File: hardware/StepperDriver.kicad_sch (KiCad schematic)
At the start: 17 parts, among them J201 Conn_01x01, J202 Conn_01x01, J203 Conn_01x01, J204 Conn_01x01, U201 TMC2130-LA

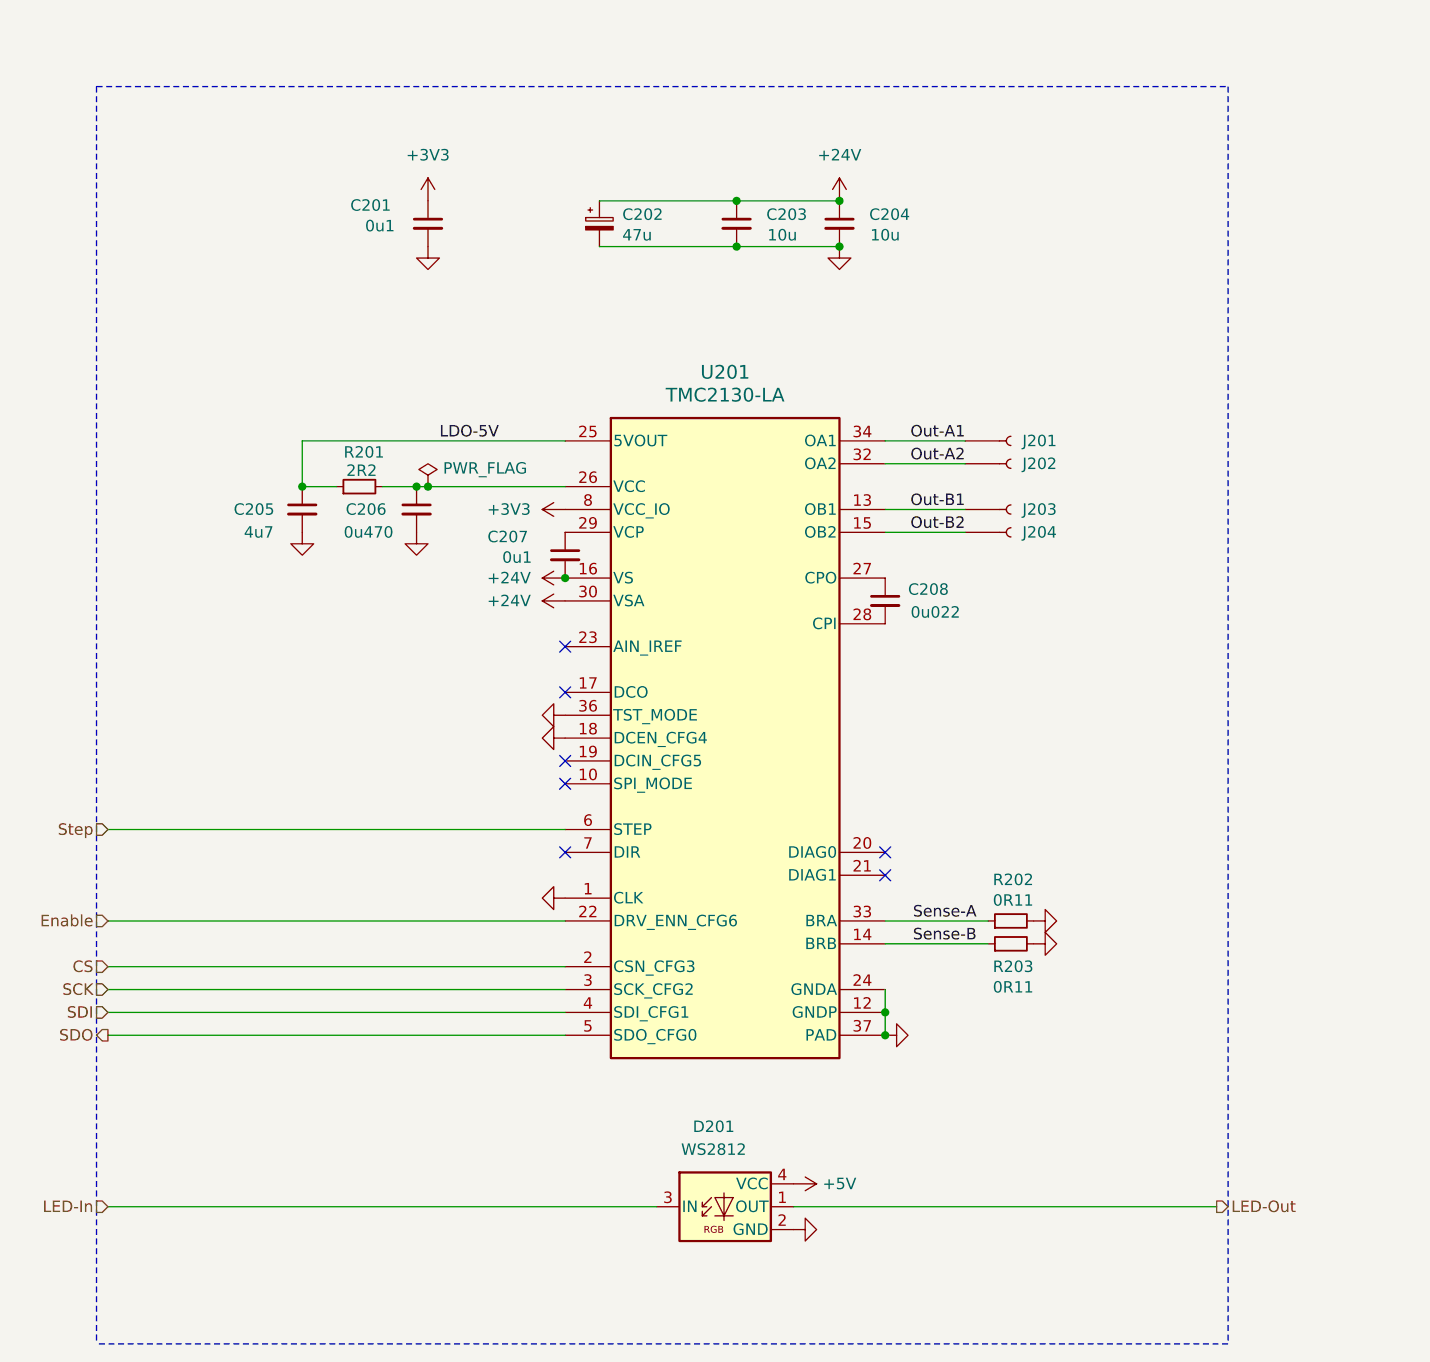
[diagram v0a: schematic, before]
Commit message: Update parts library
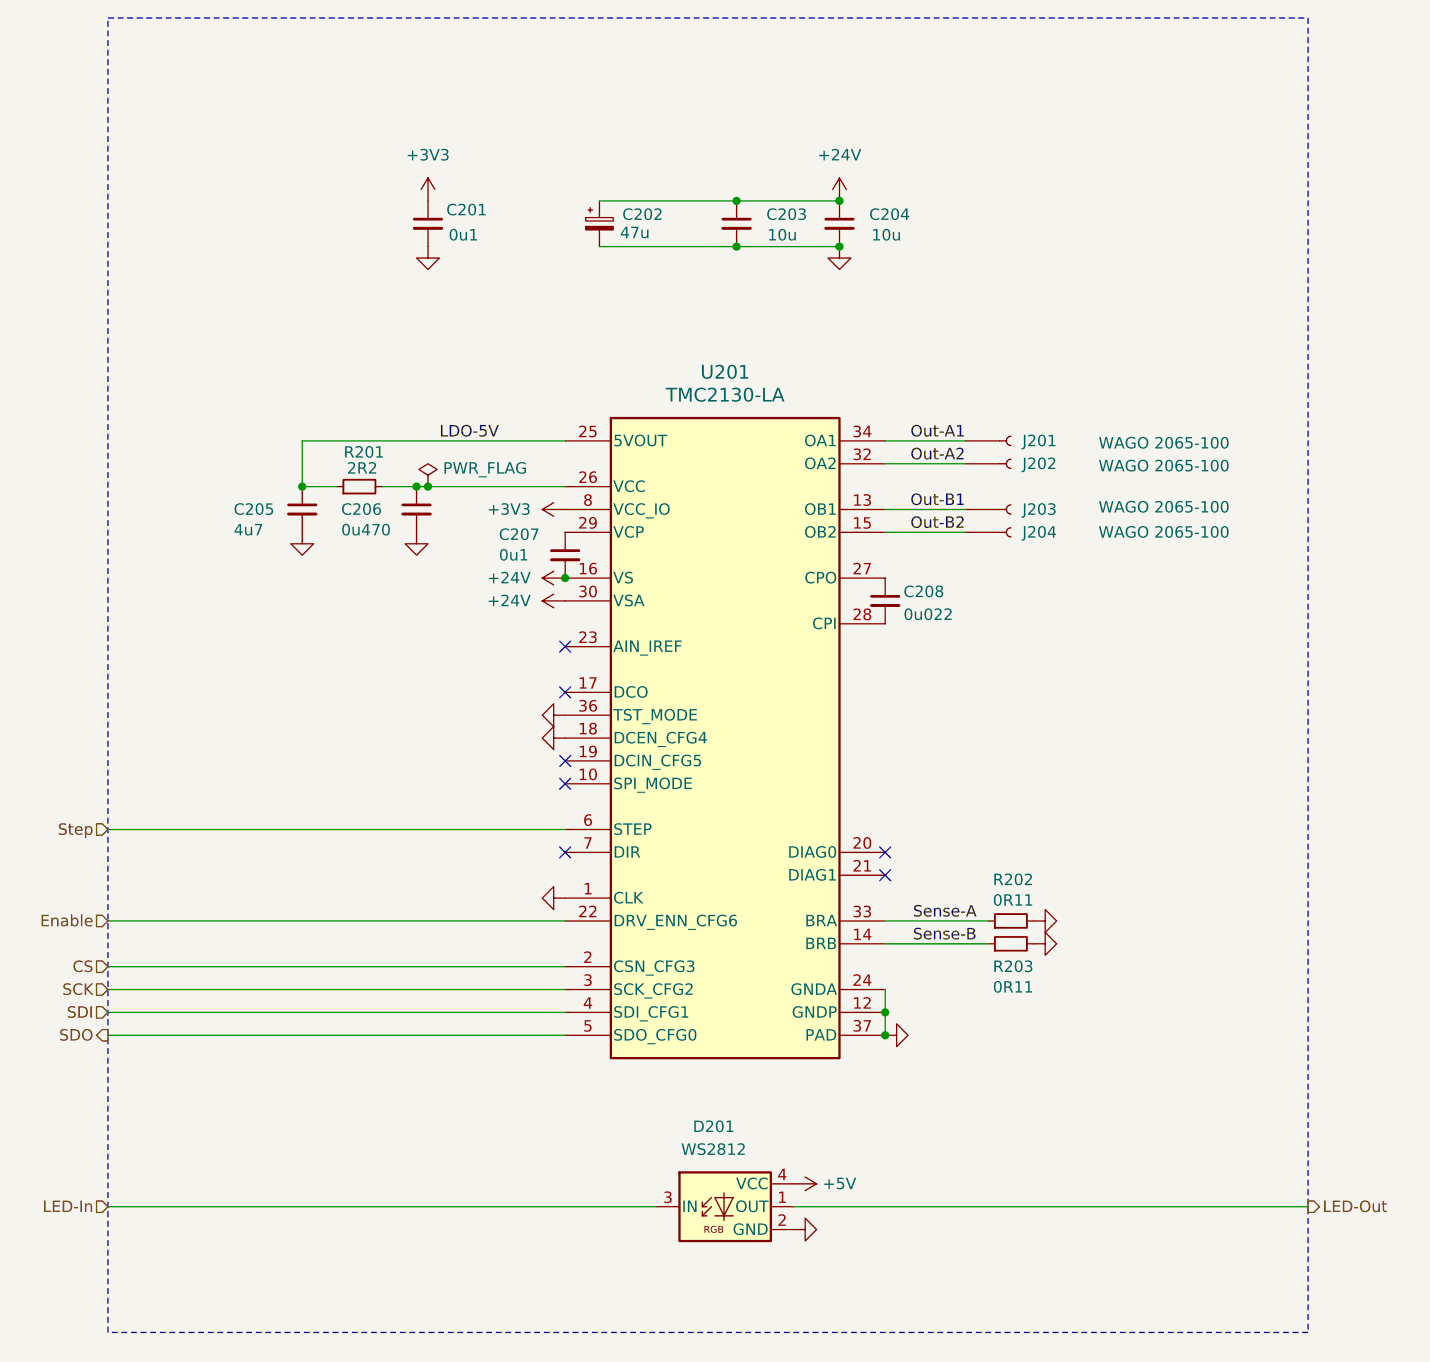
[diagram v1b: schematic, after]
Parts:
- C201, C207: footprint Capacitor_SMD:C_0603_1608Metric -> V2_Capacitor_SMD:C_0603; symbol Device:C_Small -> V2_Device:C_0603_0u1; Mouser (none) -> 810-CGA3E2X7R1H104MA
- C202: footprint Capacitor_SMD:CP_Elec_6.3x5.8 -> V2_Capacitor_SMD:CP_Elec_6.3x5.8; symbol Device:C_Polarized_Small -> V2_Device:C_Polarized_6.3x5.8_1_47u; Mouser (none) -> 667-EEE-FK1V470P
- C203, C204: footprint Capacitor_SMD:C_1210_3225Metric -> V2_Capacitor_SMD:C_1210; symbol Device:C_Small -> V2_Device:C_1210_10u; Mouser (none) -> 810-CNA6P1X7R1H106K2; Rating (none) -> 50V
- C205: footprint Capacitor_SMD:C_0603_1608Metric -> V2_Capacitor_SMD:C_0603; symbol Device:C_Small -> V2_Device:C_0603_4u7; Mouser (none) -> 603-CC603KRX5R6BB475
- C206: footprint Capacitor_SMD:C_0603_1608Metric -> V2_Capacitor_SMD:C_0603; symbol Device:C_Small -> V2_Device:C_0603_0u470; Mouser (none) -> 603-CC0603JR6BB474
- C208: footprint Capacitor_SMD:C_0603_1608Metric -> V2_Capacitor_SMD:C_0603; symbol Device:C_Small -> V2_Device:C_0603_0u022; Mouser (none) -> 603-CC603KPX7R9BB223
- J201, J202, J203, J204: value Conn_01x01 -> WAGO 2065-100
- R201: footprint Resistor_SMD:R_0603_1608Metric -> V2_Resistor_SMD:R_0603; symbol Device:R_Small -> V2_Device:R_0603_2R2; Mouser (none) -> 71-RCS06032R20JNEA
- R202, R203: footprint Resistor_SMD:R_0805_2012Metric -> V2_Resistor_SMD:R_0805; symbol Device:R_Small -> V2_Device:R_0805_0R11; Mouser (none) -> 667-ERJ-6DSFR11V
